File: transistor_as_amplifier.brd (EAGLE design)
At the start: 32.6 x 25.4 mm, 12 parts, among them T1 BC547N

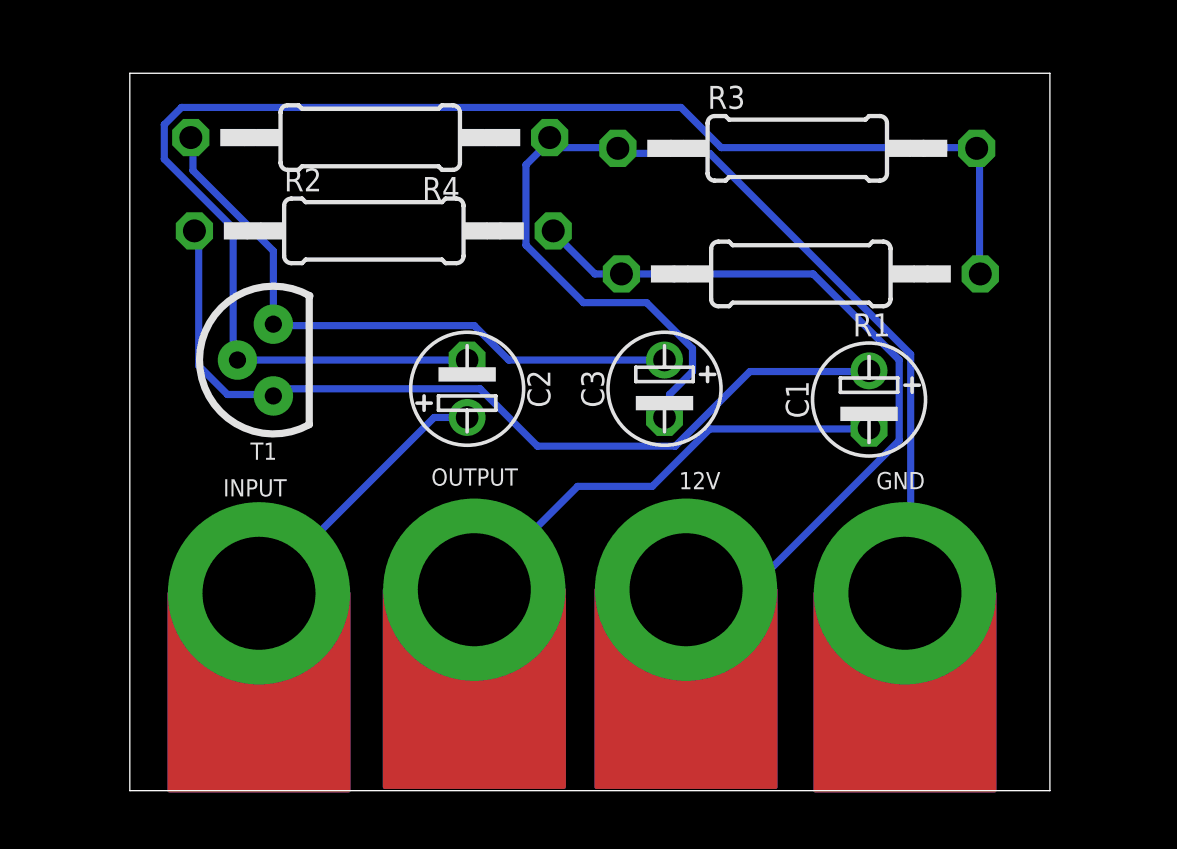
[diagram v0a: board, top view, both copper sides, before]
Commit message: updte
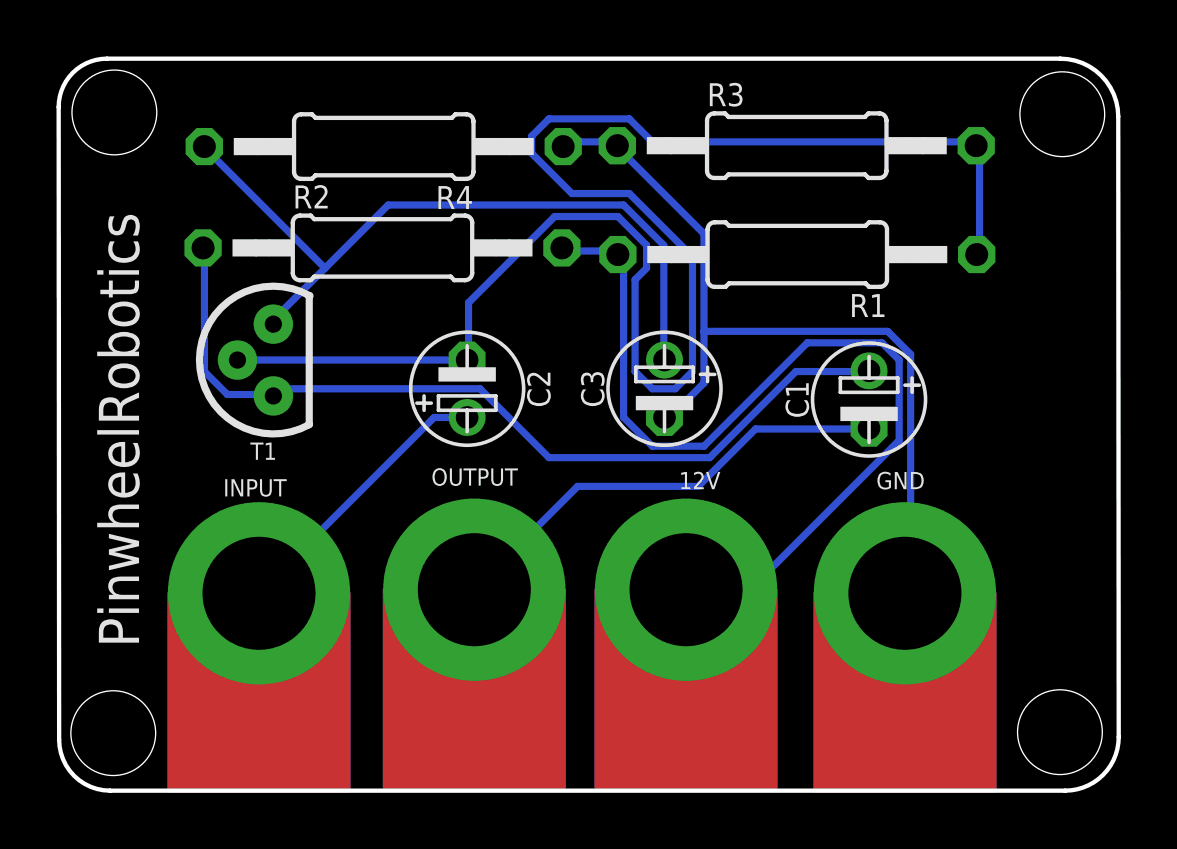
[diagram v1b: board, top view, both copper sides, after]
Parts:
- moved R1 0.70 mm to (23.6, 19.0)
- moved R2 0.68 mm to (8.94, 19.2)
- moved R4 0.57 mm to (8.99, 22.8)
- moved R3 0.10 mm to (23.6, 22.8)
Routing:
- net GND: track 39.1 -> 29.8 mm
- net N$3: track 51.7 -> 57.6 mm
- net 12V: track 26.7 -> 32.6 mm
- net N$1: track 22.2 -> 26.4 mm
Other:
- board size 32.6 x 25.4 mm -> 37.5 x 25.9 mm
- board text added: "PinwheelRobotics"
- board text added: "care@pinwheel"
